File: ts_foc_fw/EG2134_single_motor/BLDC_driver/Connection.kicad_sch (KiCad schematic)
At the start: 0 parts

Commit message: 原理图移植完成,PCB还没有布局
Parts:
- added CN1: XT30PW-M, BLDC_Drive_Tsfoc:XT30PW-M30.G.Y, symbol BLDC_Drive_Tsfoc:XT30PW-M
- added CN2: MR30PW-M30.G.Y, BLDC_Drive_Tsfoc:MR30PW-M30.G.Y, symbol BLDC_Drive_Tsfoc:MR30PW-M30.G.Y
- added CN3: WAFER-GH1.25-10PWB, BLDC_Drive_Tsfoc:WAFER-GH1.25-10PWB, symbol BLDC_Drive_Tsfoc:WAFER-GH1.25-10PWB
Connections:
- new net +12V: CN1.2 (+)
- new net GND: CN1.1 (-), CN1.3, CN1.4, CN2.4, CN2.5, CN3.1, CN3.11, CN3.12, CN3.2, CN3.3, CN3.4, CN3.5, CN3.6, CN3.7, CN3.8
- new net M0_OUT1_CS: CN3.10
- new net M0_OUT1_N: CN2.3
- new net M0_OUT2_CS: CN3.9
- new net M0_OUT2_N: CN2.2
- new net M0_OUT3: CN2.1
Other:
- note added: "Connection"

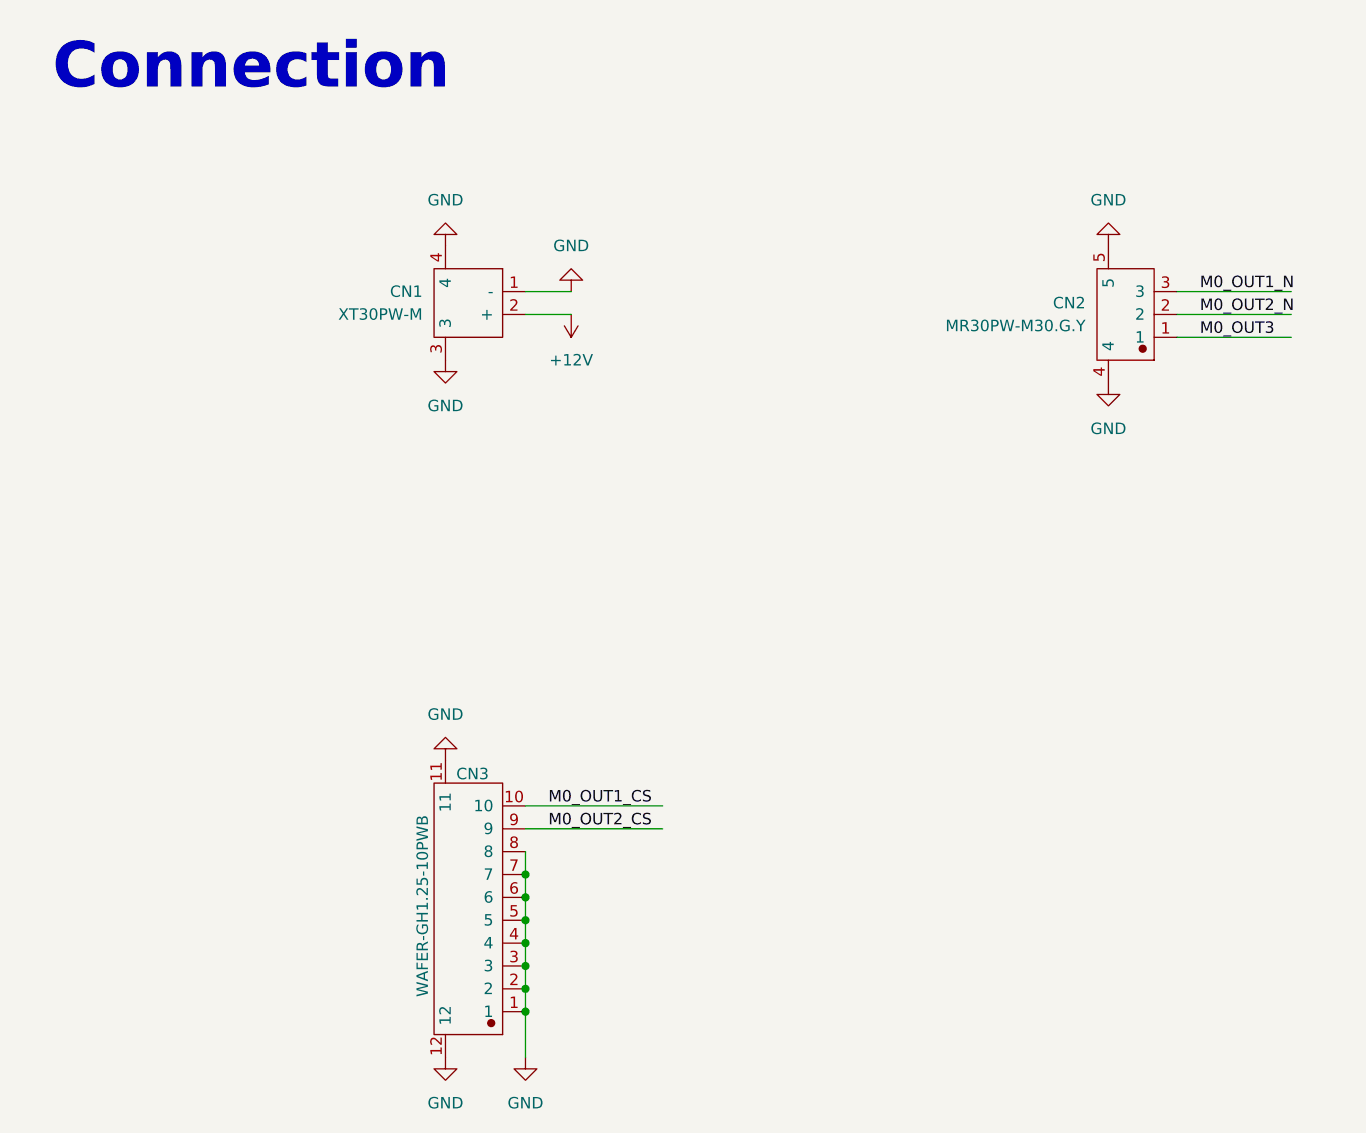
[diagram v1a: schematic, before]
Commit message: PCB_layout_ing
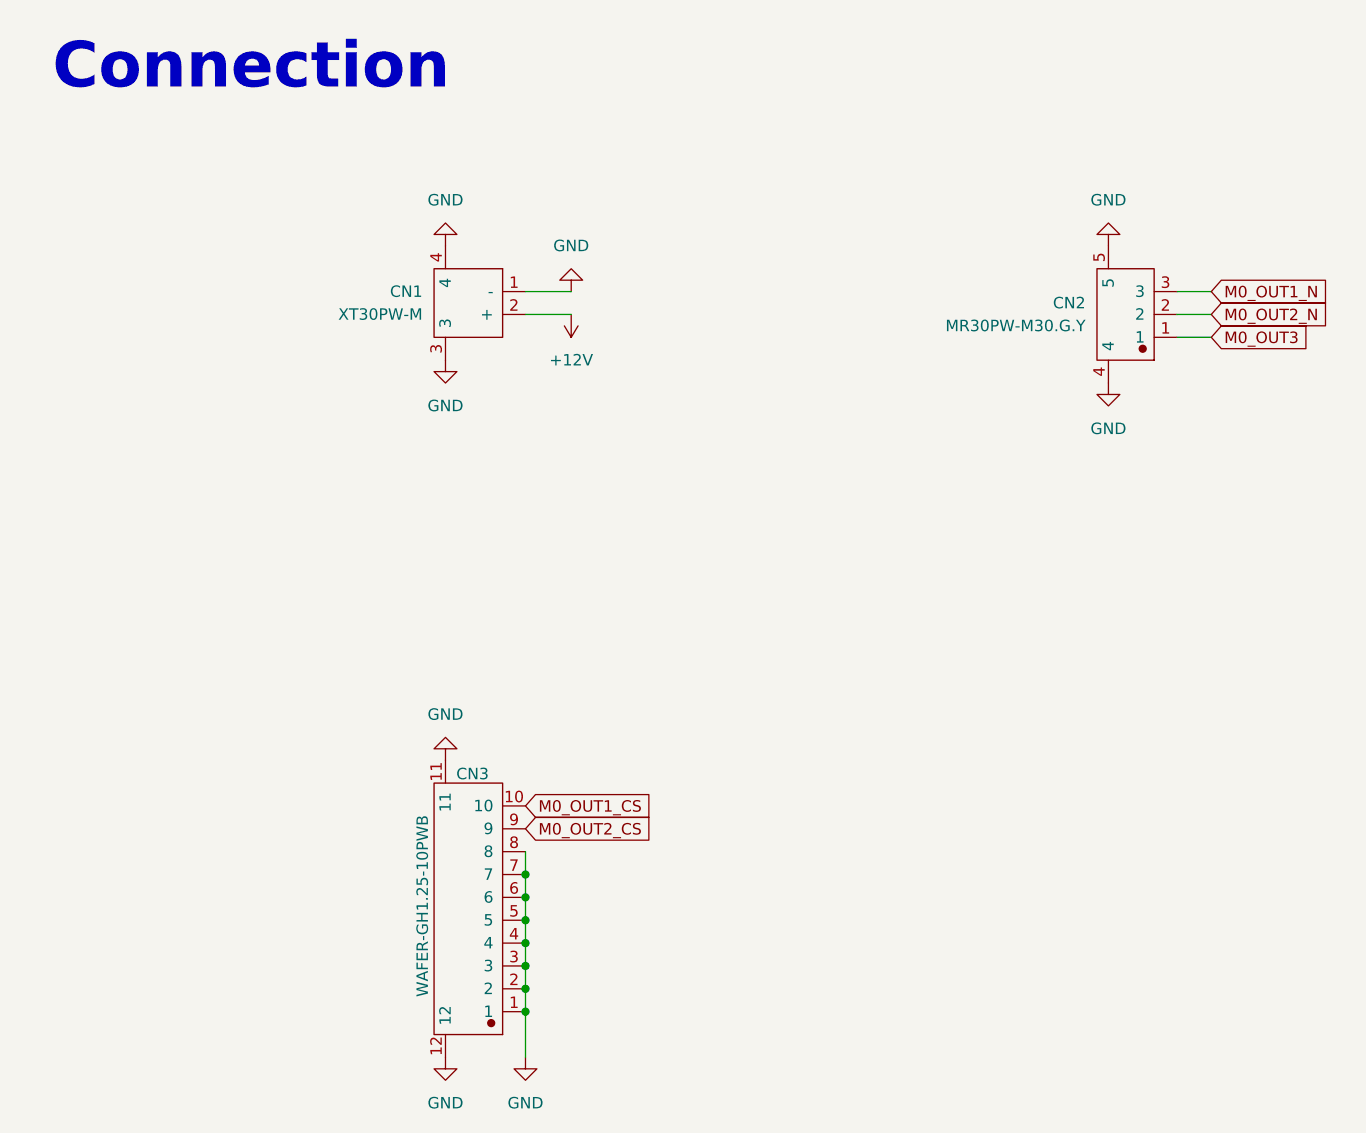
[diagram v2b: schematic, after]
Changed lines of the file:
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@@
 	(wire
 		(pts
-			(xy 138.43 49.53) (xy 151.13 49.53)
-		)
-		(stroke
-			(width 0)
-			(type default)
-		)
-	)
-	(wire
-		(pts
-			(xy 138.43 44.45) (xy 151.13 44.45)
-		)
-		(stroke
-			(width 0)
-			(type default)
-		)
-	)
-	(wire
-		(pts
-			(xy 66.04 104.14) (xy 81.28 104.14)
+			(xy 138.43 49.53) (xy 142.24 49.53)
+		)
+		(stroke
+			(width 0)
+			(type default)
+		)
+	)
+	(wire
+		(pts
+			(xy 138.43 44.45) (xy 142.24 44.45)
 		)
 		(stroke
@@
 	(wire
 		(pts
-			(xy 66.04 101.6) (xy 81.28 101.6)
-		)
-		(stroke
-			(width 0)
-			(type default)
-		)
-	)
-	(wire
-		(pts
 			(xy 66.04 109.22) (xy 66.04 111.76)
 		)
@@
 	(wire
 		(pts
-			(xy 138.43 46.99) (xy 151.13 46.99)
+			(xy 138.43 46.99) (xy 142.24 46.99)
 		)
 		(stroke
@@
 		)
 	)
-	(label "M0_OUT1_N"
-		(at 140.97 44.45 0)
-		(fields_autoplaced yes)
-		(effects
-			(font
-				(size 1.27 1.27)
-			)
-			(justify left bottom)
-		)
-	)
-	(label "M0_OUT2_N"
-		(at 140.97 46.99 0)
-		(fields_autoplaced yes)
-		(effects
-			(font
-				(size 1.27 1.27)
-			)
-			(justify left bottom)
-		)
-	)
-	(label "M0_OUT2_CS"
-		(at 68.58 104.14 0)
-		(fields_autoplaced yes)
-		(effects
-			(font
-				(size 1.27 1.27)
-			)
-			(justify left bottom)
-		)
-	)
-	(label "M0_OUT3"
-		(at 140.97 49.53 0)
-		(fields_autoplaced yes)
-		(effects
-			(font
-				(size 1.27 1.27)
-			)
-			(justify left bottom)
-		)
-	)
-	(label "M0_OUT1_CS"
-		(at 68.58 101.6 0)
-		(fields_autoplaced yes)
-		(effects
-			(font
-				(size 1.27 1.27)
-			)
-			(justify left bottom)
-		)
-	)
+	(global_label "M0_OUT1_N"
+		(shape input)
+		(at 142.24 44.45 0)
+		(fields_autoplaced yes)
+		(effects
+			(font
+				(size 1.27 1.27)
+			)
+			(justify left)
+		)
+		(property "Intersheetrefs" "${INTERSHEET_REFS}"
+			(at 155.9899 44.45 0)
+			(effects
+				(font
+					(size 1.27 1.27)
+				)
+				(justify left)
+				(hide yes)
+			)
+		)
+	)
+	(global_label "M0_OUT2_CS"
+		(shape input)
+		(at 66.04 104.14 0)
+		(fields_autoplaced yes)
+		(effects
+			(font
+				(size 1.27 1.27)
+			)
+			(justify left)
+		)
+		(property "Intersheetrefs" "${INTERSHEET_REFS}"
+			(at 80.9389 104.14 0)
+			(effects
+				(font
+					(size 1.27 1.27)
+				)
+				(justify left)
+				(hide yes)
+			)
+		)
+	)
+	(global_label "M0_OUT3"
+		(shape input)
+		(at 142.24 49.53 0)
+		(fields_autoplaced yes)
+		(effects
+			(font
+				(size 1.27 1.27)
+			)
+			(justify left)
+		)
+		(property "Intersheetrefs" "${INTERSHEET_REFS}"
+			(at 153.6918 49.53 0)
+			(effects
+				(font
+					(size 1.27 1.27)
+				)
+				(justify left)
+				(hide yes)
+			)
+		)
+	)
+	(global_label "M0_OUT1_CS"
+		(shape input)
+		(at 66.04 101.6 0)
+		(fields_autoplaced yes)
+		(effects
+			(font
+				(size 1.27 1.27)
+			)
+			(justify left)
+		)
+		(property "Intersheetrefs" "${INTERSHEET_REFS}"
+			(at 80.9389 101.6 0)
+			(effects
+				(font
+					(size 1.27 1.27)
+				)
+				(justify left)
+				(hide yes)
+			)
+		)
+	)
+	(global_label "M0_OUT2_N"
+		(shape input)
+		(at 142.24 46.99 0)
+		(fields_autoplaced yes)
+		(effects
+			(font
+				(size 1.27 1.27)
+			)
+			(justify left)
+		)
+		(property "Intersheetrefs" "${INTERSHEET_REFS}"
+			(at 155.9899 46.99 0)
+			(effects
+				(font
+					(size 1.27 1.27)
+				)
+				(justify left)
+				(hide yes)
+			)
+		)
+	)

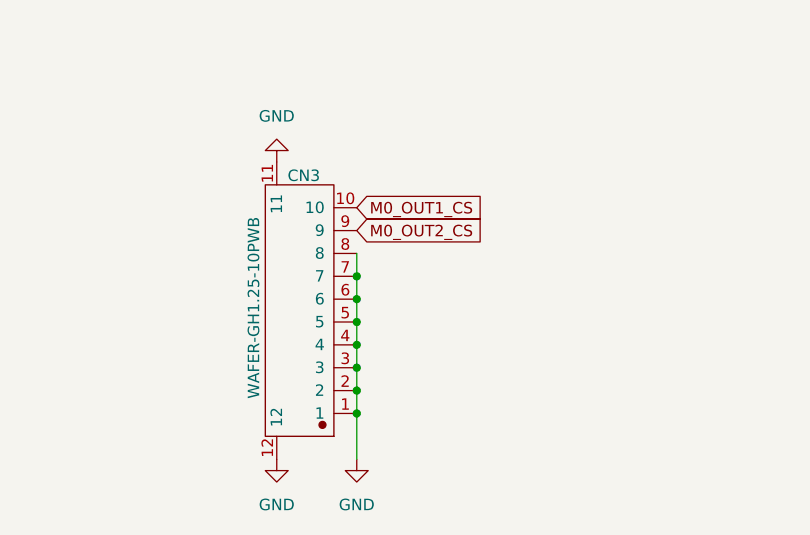
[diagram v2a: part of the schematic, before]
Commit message: 同步20241108_night
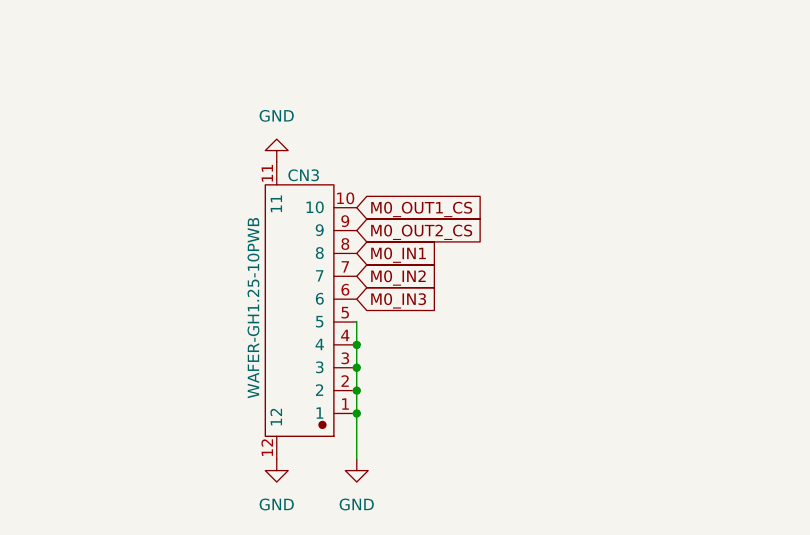
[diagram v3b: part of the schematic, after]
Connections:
- net GND: no longer CN3.6, CN3.7, CN3.8
- new net M0_IN1: CN3.8
- new net M0_IN2: CN3.7
- new net M0_IN3: CN3.6
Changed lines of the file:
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@@
-	)
-	(junction
-		(at 66.04 109.22)
-		(diameter 0)
-		(color 0 0 0 0)
 	)
 	(junction
@@
 	)
 	(junction
-		(at 66.04 114.3)
-		(diameter 0)
-		(color 0 0 0 0)
-	)
-	(junction
-		(at 66.04 111.76)
-		(diameter 0)
-		(color 0 0 0 0)
-	)
-	(junction
 		(at 66.04 116.84)
 		(diameter 0)
@@
 	(wire
 		(pts
-			(xy 66.04 111.76) (xy 66.04 114.3)
-		)
-		(stroke
-			(width 0)
-			(type default)
-		)
-	)
-	(wire
-		(pts
 			(xy 138.43 49.53) (xy 142.24 49.53)
 		)
@@
 	(wire
 		(pts
-			(xy 66.04 106.68) (xy 66.04 109.22)
-		)
-		(stroke
-			(width 0)
-			(type default)
-		)
-	)
-	(wire
-		(pts
 			(xy 66.04 46.99) (xy 71.12 46.99)
 		)
@@
 		(pts
 			(xy 66.04 114.3) (xy 66.04 116.84)
-		)
-		(stroke
-			(width 0)
-			(type default)
-		)
-	)
-	(wire
-		(pts
-			(xy 66.04 109.22) (xy 66.04 111.76)
 		)
 		(stroke
@@
 		)
 	)
+	(global_label "M0_IN1"
+		(shape input)
+		(at 66.04 106.68 0)
+		(fields_autoplaced yes)
+		(effects
+			(font
+				(size 1.27 1.27)
+			)
+			(justify left)
+		)
+		(property "Intersheetrefs" "${INTERSHEET_REFS}"
+			(at 75.7985 106.68 0)
+			(effects
+				(font
+					(size 1.27 1.27)
+				)
+				(justify left)
+				(hide yes)
+			)
+		)
+	)
+	(global_label "M0_IN3"
+		(shape input)
+		(at 66.04 111.76 0)
+		(fields_autoplaced yes)
+		(effects
+			(font
+				(size 1.27 1.27)
+			)
+			(justify left)
+		)
+		(property "Intersheetrefs" "${INTERSHEET_REFS}"
+			(at 75.7985 111.76 0)
+			(effects
+				(font
+					(size 1.27 1.27)
+				)
+				(justify left)
+				(hide yes)
+			)
+		)
+	)
 	(global_label "M0_OUT1_N"
 		(shape input)
@@
 			(effects
 				(font
+					(size 1.27 1.27)
+				)
+				(justify left)
+				(hide yes)
+			)
+		)
+	)
+	(global_label "M0_IN2"
+		(shape input)
+		(at 66.04 109.22 0)
+		(fields_autoplaced yes)
+		(effects
+			(font
+				(size 1.27 1.27)
+			)
+			(justify left)
+		)
+		(property "Intersheetrefs" "${INTERSHEET_REFS}"
+			(at 75.7985 109.22 0)
+			(effects
+				(font
